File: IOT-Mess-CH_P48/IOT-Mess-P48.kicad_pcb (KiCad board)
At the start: 2 copper layers, 29.1 x 49.8 mm, 28 parts, among them J1 Conn_02x19_Odd_Even, J10 Jumper, J11 Jumper, J12 Jumper, J14 Jumper, J2 Conn_02x19_Odd_Even, J3 Jumper_2, J6 Jumper, J7 Jumper, J8 Jumper, K1 Crystal, K32 Crystal, SW11 SW_Push, U10 USB_C_Receptacle_USB2.0_16P, U3 CH32L103C8T6, U6 ME6211C33M5

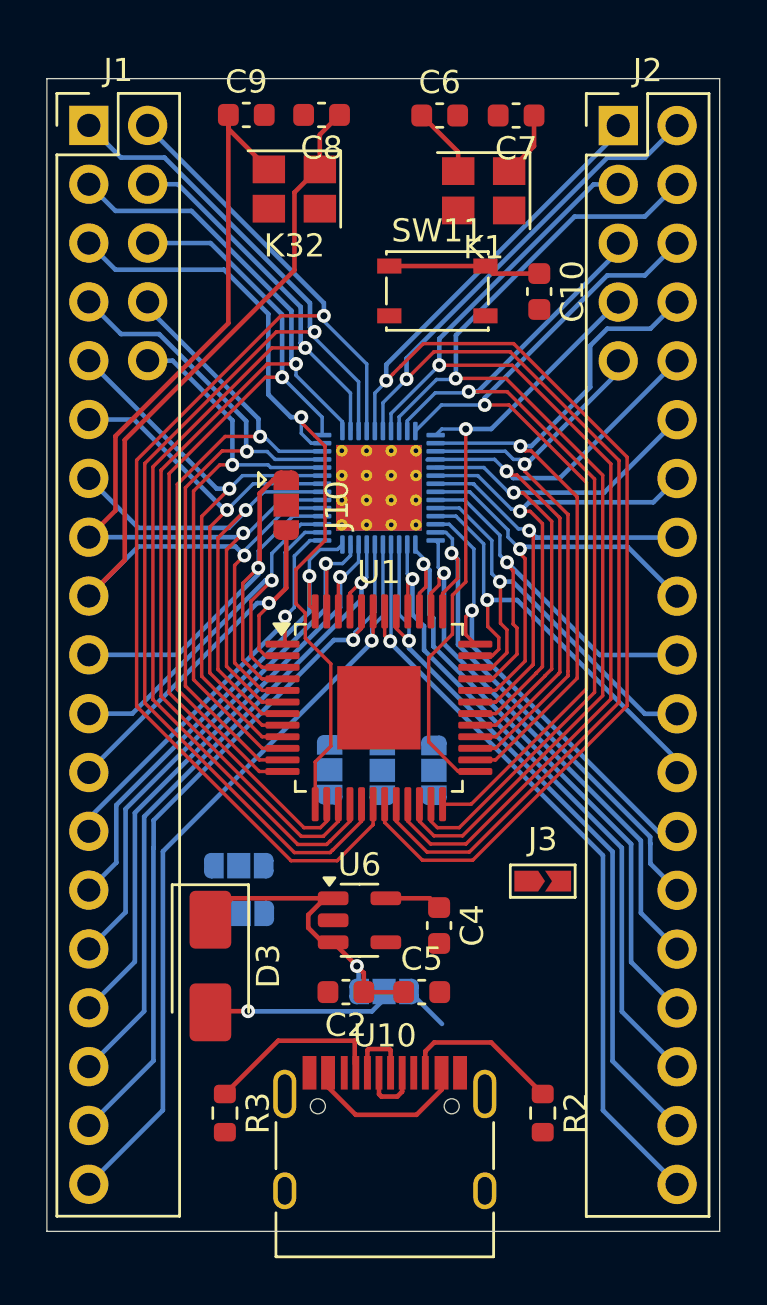
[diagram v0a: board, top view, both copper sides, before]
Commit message: did some works.
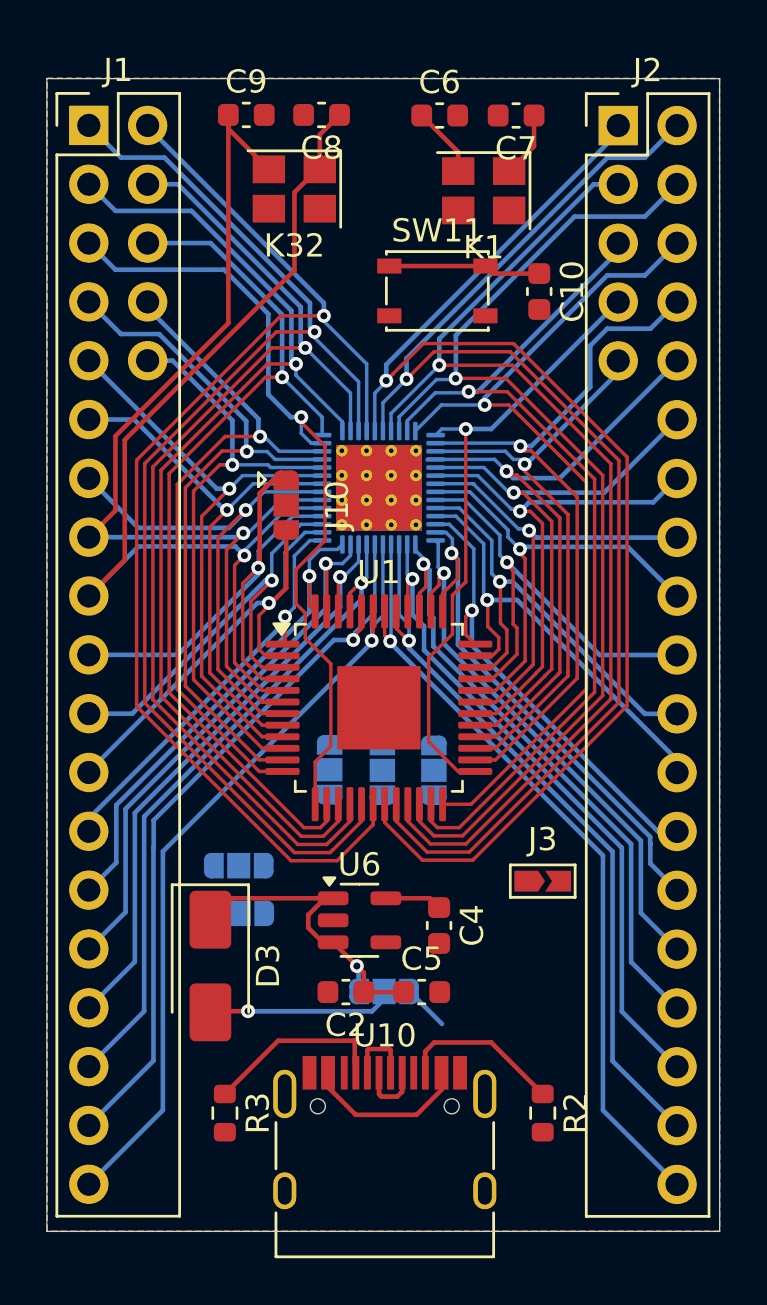
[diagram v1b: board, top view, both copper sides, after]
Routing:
- added copper zone on B.Cu, net GND
- added copper zone on F.Cu, net GND
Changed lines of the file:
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@@
 		)
 		(property "Datasheet" ""
-			(at 0 0 -90)
+			(at 0 0 270)
 			(unlocked yes)
 			(layer "B.Fab")
@@
 		)
 		(property "Description" "Solder Jumper, 3-pole, open"
-			(at 0 0 -90)
+			(at 0 0 270)
 			(unlocked yes)
 			(layer "B.Fab")
@@
 		)
 		(property "Datasheet" ""
-			(at 0 0 -90)
+			(at 0 0 270)
 			(unlocked yes)
 			(layer "B.Fab")
@@
 		)
 		(property "Description" "Solder Jumper, 3-pole, open"
-			(at 0 0 -90)
+			(at 0 0 270)
 			(unlocked yes)
 			(layer "B.Fab")
@@
 		)
 		(property "Datasheet" ""
-			(at 0 0 -90)
+			(at 0 0 270)
 			(unlocked yes)
 			(layer "B.Fab")
@@
 		)
 		(property "Description" "Solder Jumper, 3-pole, open"
-			(at 0 0 -90)
+			(at 0 0 270)
 			(unlocked yes)
 			(layer "B.Fab")
@@
 		(net 61)
 	)
+	(zone
+		(net 2)
+		(net_name "GND")
+		(layers "F.Cu" "B.Cu")
+		(hatch edge 0.5)
+		(connect_pads
+			(clearance 0.5)
+		)
+		(min_thickness 0.25)
+		(filled_areas_thickness no)
+		(fill yes
+			(thermal_gap 0.5)
+			(thermal_bridge_width 0.5)
+		)
+		(polygon
+			(pts
+				(xy 189.55 73.29) (xy 218.58 73.3) (xy 218.59 123.07) (xy 189.55 123.05)
+			)
+		)
+	)
 	(embedded_fonts no)
